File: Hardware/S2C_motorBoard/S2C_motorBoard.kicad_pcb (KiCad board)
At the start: 4 copper layers, 38 x 43 mm, 40 parts, among them J101 UART, J102 Conn_ST_STDC14, J103 USB_C_Receptacle_USB2.0_16P, J201 Moteur, J301 Moteur, U101 WPME-VDLM, U102 STM32G431CBUx, U103 USBLC6-2SC6, U201 MIC4606, U202 FDMQ86530L, U301 MIC4606, U302 FDMQ86530L

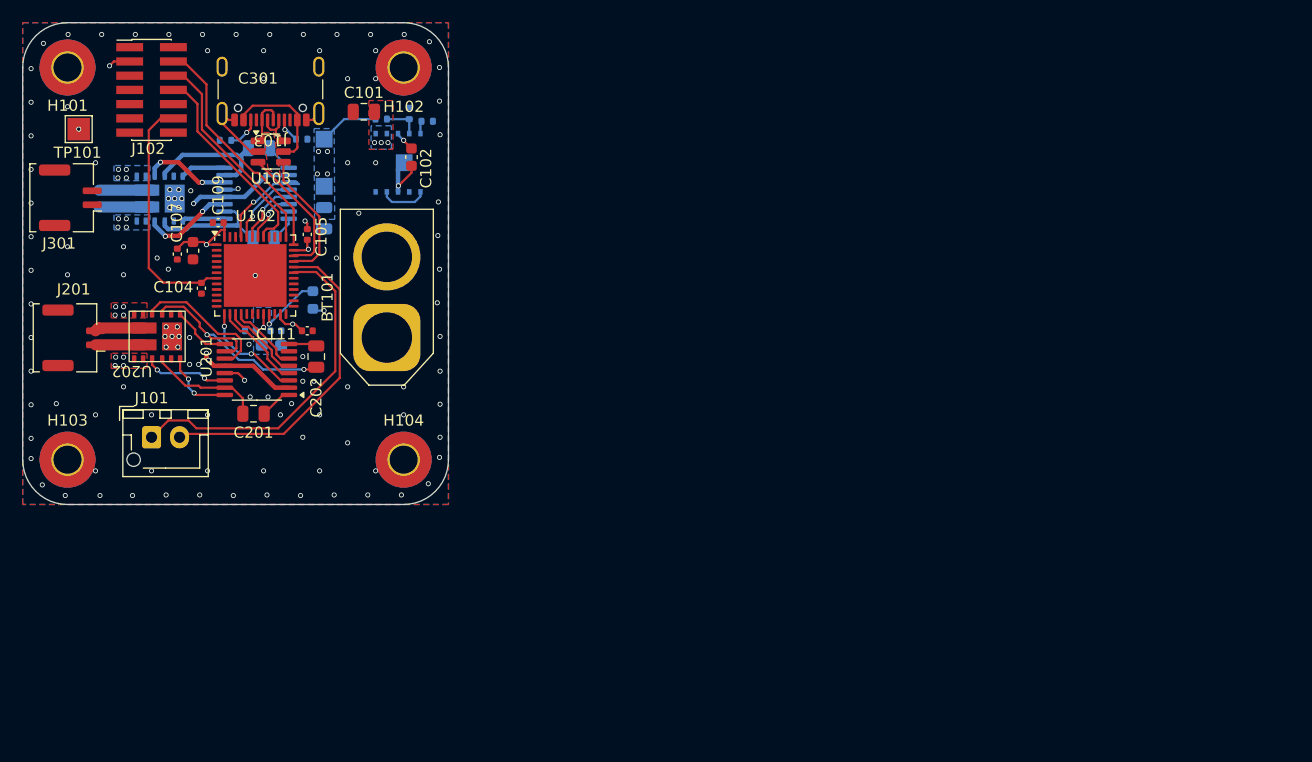
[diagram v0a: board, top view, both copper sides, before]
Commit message: PCB update
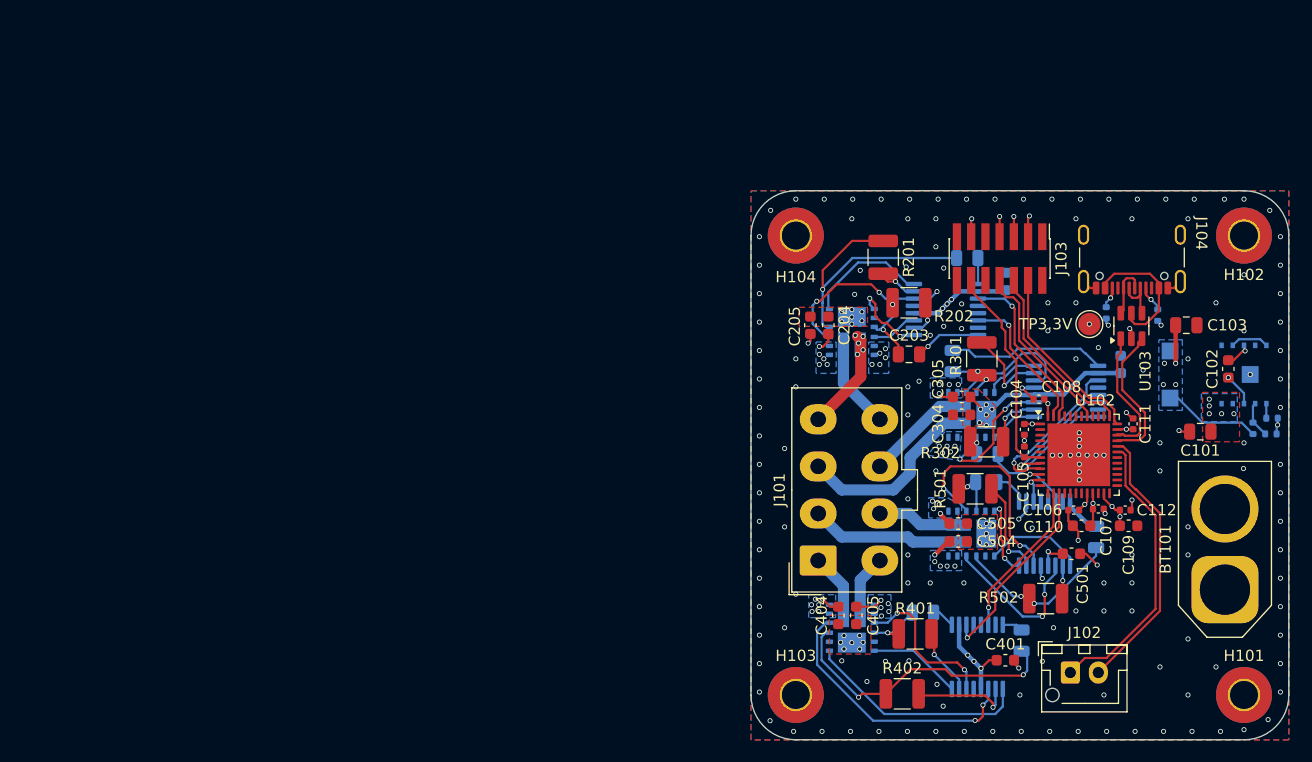
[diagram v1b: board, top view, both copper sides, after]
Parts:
- removed J201, J301: Moteur, Connector_Molex:Molex_CLIK-Mate_502382-0270_1x02-1MP_P1.25mm_Vertical
- removed L101: 39n, Inductor_SMD:L_0603_1608Metric
- removed TP101: 3.3V, TestPoint:TestPoint_Pad_2.0x2.0mm
- added C203: 1u, Capacitor_SMD:C_0805_2012Metric, F.Cu at (165.1, 69.6)
- added C204: 10u, Capacitor_SMD:C_0603_1608Metric, F.Cu at (157.9, 67.0)
- added C205: 10u, Capacitor_SMD:C_0603_1608Metric, F.Cu at (156.3, 67.0)
- added C303: 1u, Capacitor_SMD:C_0805_2012Metric, B.Cu at (172.1, 78.5)
- added C304: 10u, Capacitor_SMD:C_0603_1608Metric, F.Cu at (169.8, 75.0)
- added C305: 10u, Capacitor_SMD:C_0603_1608Metric, F.Cu at (169.8, 73.4)
- added C401: 2u2, Capacitor_SMD:C_0603_1608Metric, F.Cu at (173.7, 96.9)
- added C402: 1u, Capacitor_SMD:C_0805_2012Metric, B.Cu at (166.3, 92.7)
- added C403: 1u, Capacitor_SMD:C_0805_2012Metric, B.Cu at (175.2, 95.2)
- added C404: 10u, Capacitor_SMD:C_0603_1608Metric, F.Cu at (158.8, 92.9)
- added C405: 10u, Capacitor_SMD:C_0603_1608Metric, F.Cu at (160.4, 92.9)
- added C501: 2u2, Capacitor_SMD:C_0603_1608Metric, F.Cu at (179.6, 87.4)
- added C502: 1u, Capacitor_SMD:C_0805_2012Metric, B.Cu at (172.0, 81.0)
- added C503: 1u, Capacitor_SMD:C_0805_2012Metric, B.Cu at (181.8, 85.9)
- added C504: 10u, Capacitor_SMD:C_0603_1608Metric, F.Cu at (169.5, 86.3)
- added C505: 10u, Capacitor_SMD:C_0603_1608Metric, F.Cu at (169.5, 84.7)
- added J104: USB_C_Receptacle_USB2.0_16P, Connector_USB:USB_C_Receptacle_GCT_USB4105-xx-A_16P_TopMnt_Horizontal, F.Cu at (185.0, 60.0)
- added R201: 0R3, Resistor_SMD:R_1210_3225Metric, F.Cu at (162.8, 60.9)
- added R202: 0R3, Resistor_SMD:R_1210_3225Metric, F.Cu at (165.1, 65.0)
- added R301: 0R3, Resistor_SMD:R_1210_3225Metric, F.Cu at (171.6, 70.0)
- added R302: 0R3, Resistor_SMD:R_1210_3225Metric, F.Cu at (172.0, 77.4)
- added R401: 0R3, Resistor_SMD:R_1210_3225Metric, F.Cu at (165.7, 94.5)
- added R402: 0R3, Resistor_SMD:R_1210_3225Metric, F.Cu at (164.5, 99.9)
- added R501: 0R3, Resistor_SMD:R_1210_3225Metric, F.Cu at (171.0, 81.6)
- added R502: 0R3, Resistor_SMD:R_1210_3225Metric, F.Cu at (177.3, 91.4)
- added TP3.3V: 3.3V, TestPoint:TestPoint_Pad_D2.0mm, F.Cu at (181.2, 66.9)
- added U401: MIC4606, Package_SO:TSSOP-16_4.4x5mm_P0.65mm, B.Cu at (171.2, 96.6)
- added U402: FDMQ86530L, CustomLibrary:FDMQ86530L, B.Cu at (160.0, 94.0)
- added U501: MIC4606, Package_SO:TSSOP-16_4.4x5mm_P0.65mm, B.Cu at (177.2, 85.6)
- added U502: FDMQ86530L, CustomLibrary:FDMQ86530L, B.Cu at (170.7, 85.6)
- C103, C108: moved to F.Cu
- C104: value 10n -> 100n
- C105: value 100n -> 10n
- C106: value 1u -> 100n; footprint Capacitor_SMD:C_0603_1608Metric_Pad1.08x0.95mm_HandSolder -> Capacitor_SMD:C_0402_1005Metric; moved to F.Cu
- C109: value 100n -> 10u; footprint Capacitor_SMD:C_0402_1005Metric -> Capacitor_SMD:C_0603_1608Metric
- C110: value 100n -> 1u; footprint Capacitor_SMD:C_0402_1005Metric -> Capacitor_SMD:C_0603_1608Metric; moved to F.Cu
- C112: value 10u -> 100n; footprint Capacitor_SMD:C_0603_1608Metric -> Capacitor_SMD:C_0402_1005Metric
- C201: value 1u -> 2u2; footprint Capacitor_SMD:C_0805_2012Metric -> Capacitor_SMD:C_0603_1608Metric; moved to B.Cu
- C202, U201, U202: moved to B.Cu
- C301: value 1u -> 2u2; footprint Capacitor_SMD:C_0805_2012Metric -> Capacitor_SMD:C_0603_1608Metric
- J101: value UART -> Conn_02x04_Odd_Even; footprint Connector_JST:JST_XH_B2B-XH-AM_1x02_P2.50mm_Vertical -> Connector_Molex:Molex_Mini-Fit_Jr_5566-08A_2x04_P4.20mm_Vertical
- J102: value Conn_ST_STDC14 -> UART; footprint Connector_PinHeader_1.27mm:PinHeader_2x07_P1.27mm_Vertical_SMD -> Connector_JST:JST_XH_B2B-XH-AM_1x02_P2.50mm_Vertical
- J103: value USB_C_Receptacle_USB2.0_16P -> Conn_ST_STDC14; footprint Connector_USB:USB_C_Receptacle_GCT_USB4105-xx-A_16P_TopMnt_Horizontal -> Connector_PinHeader_1.27mm:PinHeader_2x07_P1.27mm_Vertical_SMD
- moved H101 119.0 mm to (195.0, 100.0)
- moved J102 97.1 mm to (179.5, 98.0)
- moved C112 86.4 mm to (184.4, 83.5), turned to 0 degrees
- moved C109 85.6 mm to (184.7, 84.9), turned to 0 degrees
- moved C107 85.3 mm to (182.0, 83.4), turned to 0 degrees
- moved R102 82.6 mm to (195.8, 76.2), turned to 90 degrees
- moved R103 82.0 mm to (197.4, 76.7), turned to 0 degrees
- moved R105 80.1 mm to (182.7, 65.9), turned to 90 degrees
- moved C101 79.9 mm to (191.1, 76.5)
- moved R101 79.9 mm to (197.5, 75.3)
- moved C301 79.3 mm to (184.0, 70.5), turned to 90 degrees
- moved U103 78.4 mm to (184.9, 67.1), turned to 90 degrees
- moved BT101 78.1 mm to (193.3, 90.6)
- moved R104 78.0 mm to (187.3, 66.1), turned to -90 degrees
- moved U101 77.8 mm to (192.5, 71.4)
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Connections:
- BT101 pad 1: +7.5V -> GND
- BT101 pad 2: GND -> +7.5V
- C104 pad 1: /NRST -> +3.3V
- C105 pad 1: +3.3V -> /NRST
- C106 pad 1: +3.3VA -> +3.3V
- C108 pad 1: +3.3VA -> +3.3V
- C110 pad 1: +3.3VA -> +3.3V
- C201 pad 1: Net-(U201-BHB) -> +7.5V
- C201 pad 2: /Motor1/ARM_B_mes -> GND
- C202 pad 1: /Motor1/ARM_A_mes -> Net-(U201-BHB)
- C202 pad 2: Net-(U201-AHB) -> /Motor1/ARM_B_mes
- C301 pad 1: Net-(U301-BHB) -> +7.5V
- C301 pad 2: /Motor2/ARM_B_mes -> GND
- C302 pad 1: /Motor2/ARM_A_mes -> Net-(U301-BHB)
- C302 pad 2: Net-(U301-AHB) -> /Motor2/ARM_B_mes
- J101 pad 1: /TX -> /M4_ARM_B
- J101 pad 2: /RX -> /M3_ARM_B
- J102 pad 1: unconnected-(J102-NC-Pad1) -> /TX
- J102 pad 2: unconnected-(J102-NC-Pad2) -> /RX
- R104 pad 1: Net-(J103-CC1) -> Net-(J104-CC1)
- R105 pad 2: Net-(J103-CC2) -> Net-(J104-CC2)
- U102 pad 10: unconnected-(U102-PA2-Pad10) -> /M3_In_A
- U102 pad 11: unconnected-(U102-PA3-Pad11) -> /M3_In_B
- U102 pad 13: /M1_In_B_H -> unconnected-(U102-PA5-Pad13)
- U102 pad 14: /M1_In_B_L -> /M4_In_A
- U102 pad 15: /M1_In_A_L -> /M4_In_B
- U102 pad 16: /M1_In_A_H -> unconnected-(U102-PC4-Pad16)
- U102 pad 20: +3.3VA -> +3.3V
- U102 pad 21: +3.3VA -> +3.3V
- U102 pad 42: /M2_In_A_H -> unconnected-(U102-PB4-Pad42)
- U102 pad 43: /M2_In_A_L -> unconnected-(U102-PB5-Pad43)
- U102 pad 44: /M2_In_B_L -> unconnected-(U102-PB6-Pad44)
- U102 pad 45: /M2_In_B_H -> unconnected-(U102-PB7-Pad45)
- U102 pad 46: unconnected-(U102-PB8-Pad46) -> /M1_In_B
- U102 pad 47: unconnected-(U102-PB9-Pad47) -> /M1_In_A
- U102 pad 8: unconnected-(U102-PA0-Pad8) -> /M2_In_A
- U102 pad 9: unconnected-(U102-PA1-Pad9) -> /M2_In_B
- U103 pad 1: /D+ -> /USB_DP
- U103 pad 3: /USB_DP -> /USB_DN
- U103 pad 4: /USB_DN -> /D-
- U103 pad 6: /D- -> /D+
- U201 pad 10: /Motor1/ARM_A_mes -> Net-(U201-AHS)
- U201 pad 15: /Motor1/ARM_B_mes -> Net-(U201-BHS)
- U201 pad 3: /M1_In_B_H -> /M1_In_B
- U201 pad 4: /M1_In_B_L -> unconnected-(U201-BLI-Pad4)
- U201 pad 5: /M1_In_A_L -> unconnected-(U201-ALI-Pad5)
- U201 pad 6: /M1_In_A_H -> /M1_In_A
- U202 pad 14: /Motor1/ARM_A -> /M1_ARM_A
- U202 pad 15: /Motor1/ARM_B -> /M1_ARM_B
- U301 pad 10: /Motor2/ARM_A_mes -> Net-(U301-AHS)
- U301 pad 15: /Motor2/ARM_B_mes -> Net-(U301-BHS)
- U301 pad 3: /M2_In_B_H -> /M2_In_B
- U301 pad 4: /M2_In_B_L -> unconnected-(U301-BLI-Pad4)
- U301 pad 5: /M2_In_A_L -> unconnected-(U301-ALI-Pad5)
- U301 pad 6: /M2_In_A_H -> /M2_In_A
- U302 pad 14: /Motor2/ARM_A -> /M2_ARM_A
- U302 pad 15: /Motor2/ARM_B -> /M2_ARM_B
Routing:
- net /Motor4/ARM_A_mes: track 0.00 -> 26.1 mm, vias 0 -> 2
- net GND: track 17.3 -> 41.4 mm, vias 120 -> 211
- net /Motor4/Cmd_L_A: track 0.00 -> 24.1 mm, vias 0 -> 2
- net /Motor4/Cmd_H_A: track 0.00 -> 20.1 mm
- net /Motor3/Cmd_L_B: track 0.00 -> 20.0 mm, vias 0 -> 2
- net +7.5V: track 18.4 -> 36.9 mm, vias 20 -> 40
- net /M4_In_B: track 0.00 -> 17.5 mm, vias 0 -> 1
- net /M2_ARM_B: track 0.00 -> 16.7 mm
- net /Motor1/ARM_A_mes: track 21.5 -> 6.38 mm
- net /M1_In_B: track 0.00 -> 15.1 mm, vias 0 -> 1
- net /Motor3/ARM_A_mes: track 0.00 -> 15.1 mm, vias 0 -> 2
- net /Motor1/ARM_B_mes: track 10.2 -> 25.2 mm, vias 0 -> 1
- net /M2_In_B: track 0.00 -> 14.3 mm, vias 0 -> 1
- net /Motor3/Cmd_L_A: track 0.00 -> 14.2 mm, vias 0 -> 2
- net /M4_In_A: track 0.00 -> 14.2 mm, vias 0 -> 1
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- removed copper zone on F.Cu, net (none)
- removed copper zone on B.Cu, net +3.3VA
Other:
- board size 38 x 43 mm -> 48 x 49 mm
